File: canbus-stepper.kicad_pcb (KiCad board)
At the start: 2 copper layers, 40.3 x 40.3 mm, 63 parts, among them J1 TYPE-C USB SOCKET, J2 Motor Output, J3 CAN Daisy-Chain 1, J4 CAN Daisy-Chain 2, J5 Qwiic I2C, J6 AUX Port, J7 SFV30R-2STBE1HLF (30-Pin OLED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, J8 24V Power Input Terminal, J9 24V Power Output Terminal, Q1 AO4407A, SW1 SW_Push, SW2 SW_Push, SW3 SW_Push, SW4 SW_Push, U1 ESP32-S3-WROOM-1, U2 TMC2209, U3 AS5600-ASOT, U4 TCAN1051VDRBTQ1, U5 MP2315, U6 AP2112K-3.3TRG1, U7 USBLC6-2SC6

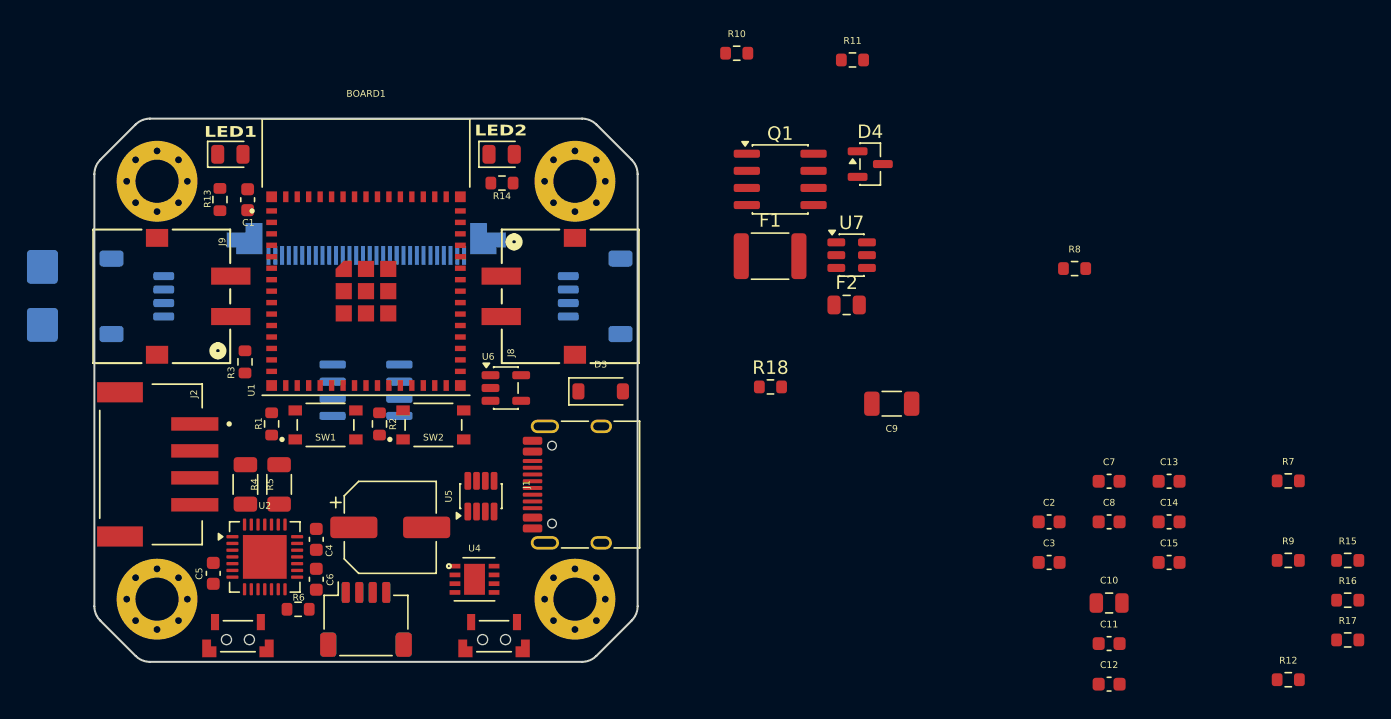
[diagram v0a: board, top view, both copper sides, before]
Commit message: chore: save PCB editor update state prior to unplaced component grouping
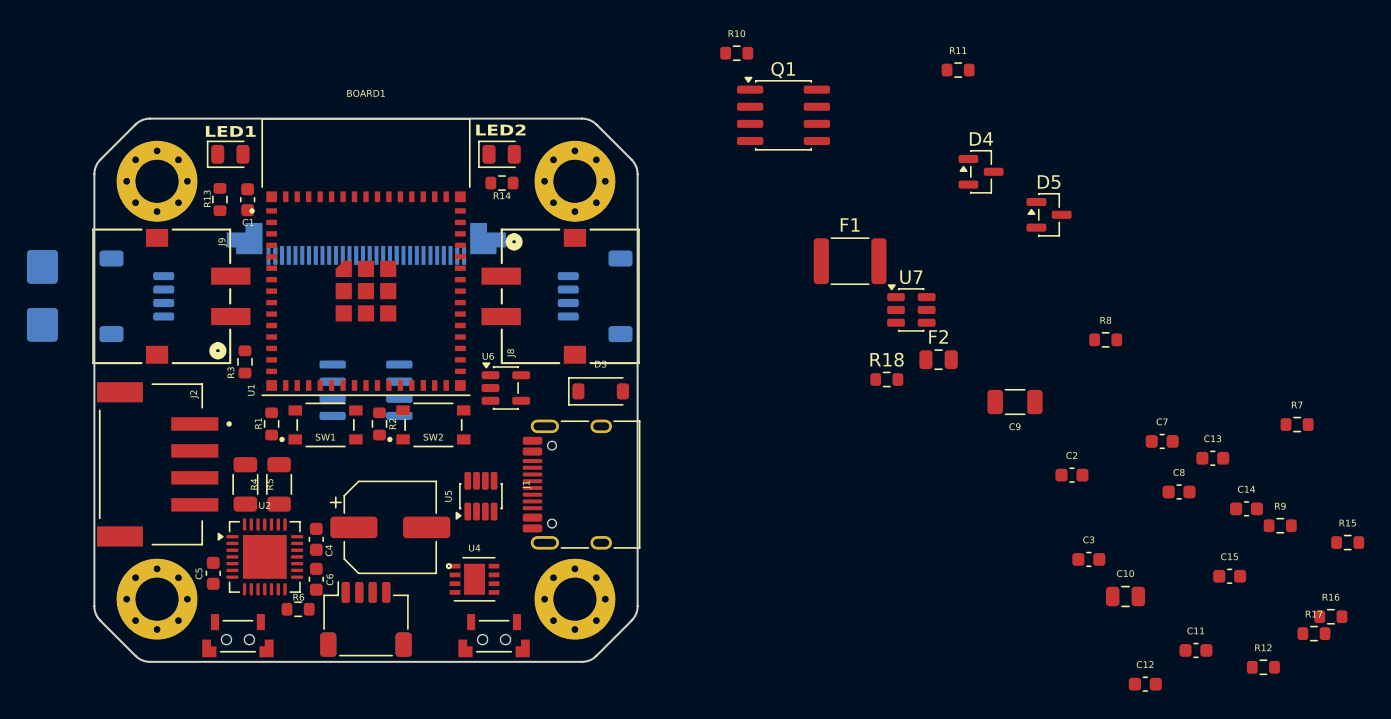
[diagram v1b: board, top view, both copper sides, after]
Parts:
- added D5: BZX84C12V, Package_TO_SOT_SMD:SOT-23, F.Cu at (199.2, 92.0)
- moved C9 9.15 mm to (196.6, 105.9)
- moved R18 8.65 mm to (187.1, 104.2)
- moved D4 8.24 mm to (194.1, 88.8)
- moved F2 7.94 mm to (191.0, 102.7)
- moved R11 7.87 mm to (192.4, 81.3)
- moved C11 6.46 mm to (210.1, 124.3)
- moved U7 6.01 mm to (189.0, 99.0)
- moved F1 5.95 mm to (184.4, 95.4)
- moved C14 5.82 mm to (213.8, 113.8)
- moved R8 5.77 mm to (203.4, 101.3)
- moved C8 5.64 mm to (208.8, 112.5)
- moved C7 4.93 mm to (207.6, 108.8)
- moved Q1 4.76 mm to (179.5, 84.6)
- moved C15 4.61 mm to (212.6, 118.8)
- moved R7 4.23 mm to (217.6, 107.5)
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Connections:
- Q1 pad 4: (no net) -> unconnected-(Q1-G-Pad4)
- Q1 pad 5: (no net) -> unconnected-(Q1-D-Pad5)
- Q1 pad 6: (no net) -> unconnected-(Q1-D-Pad6)
- Q1 pad 7: (no net) -> unconnected-(Q1-D-Pad7)
- Q1 pad 8: (no net) -> unconnected-(Q1-D-Pad8)
